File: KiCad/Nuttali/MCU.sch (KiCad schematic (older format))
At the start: 34 parts, among them J1 SWD, SW1 SW_DPST_x2, SW2 RND 210-00662, U1 STM32F411RETx, Y1 16Mhz

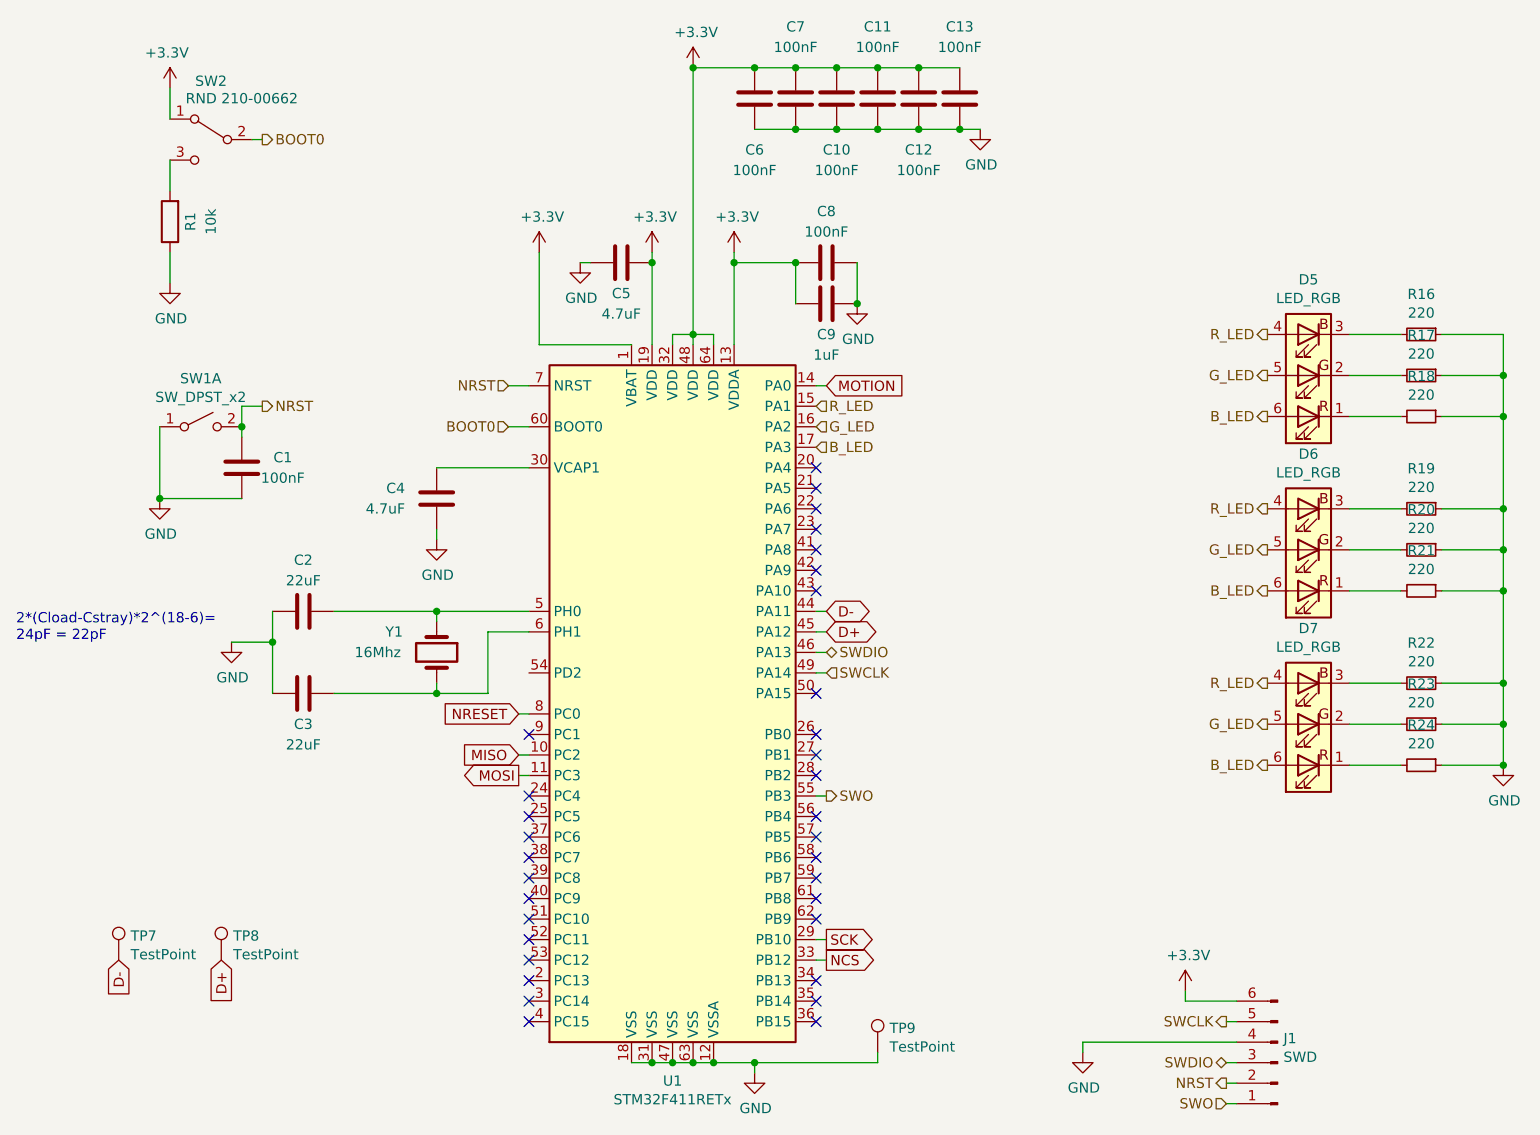
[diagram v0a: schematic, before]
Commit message: First draft of the pcb
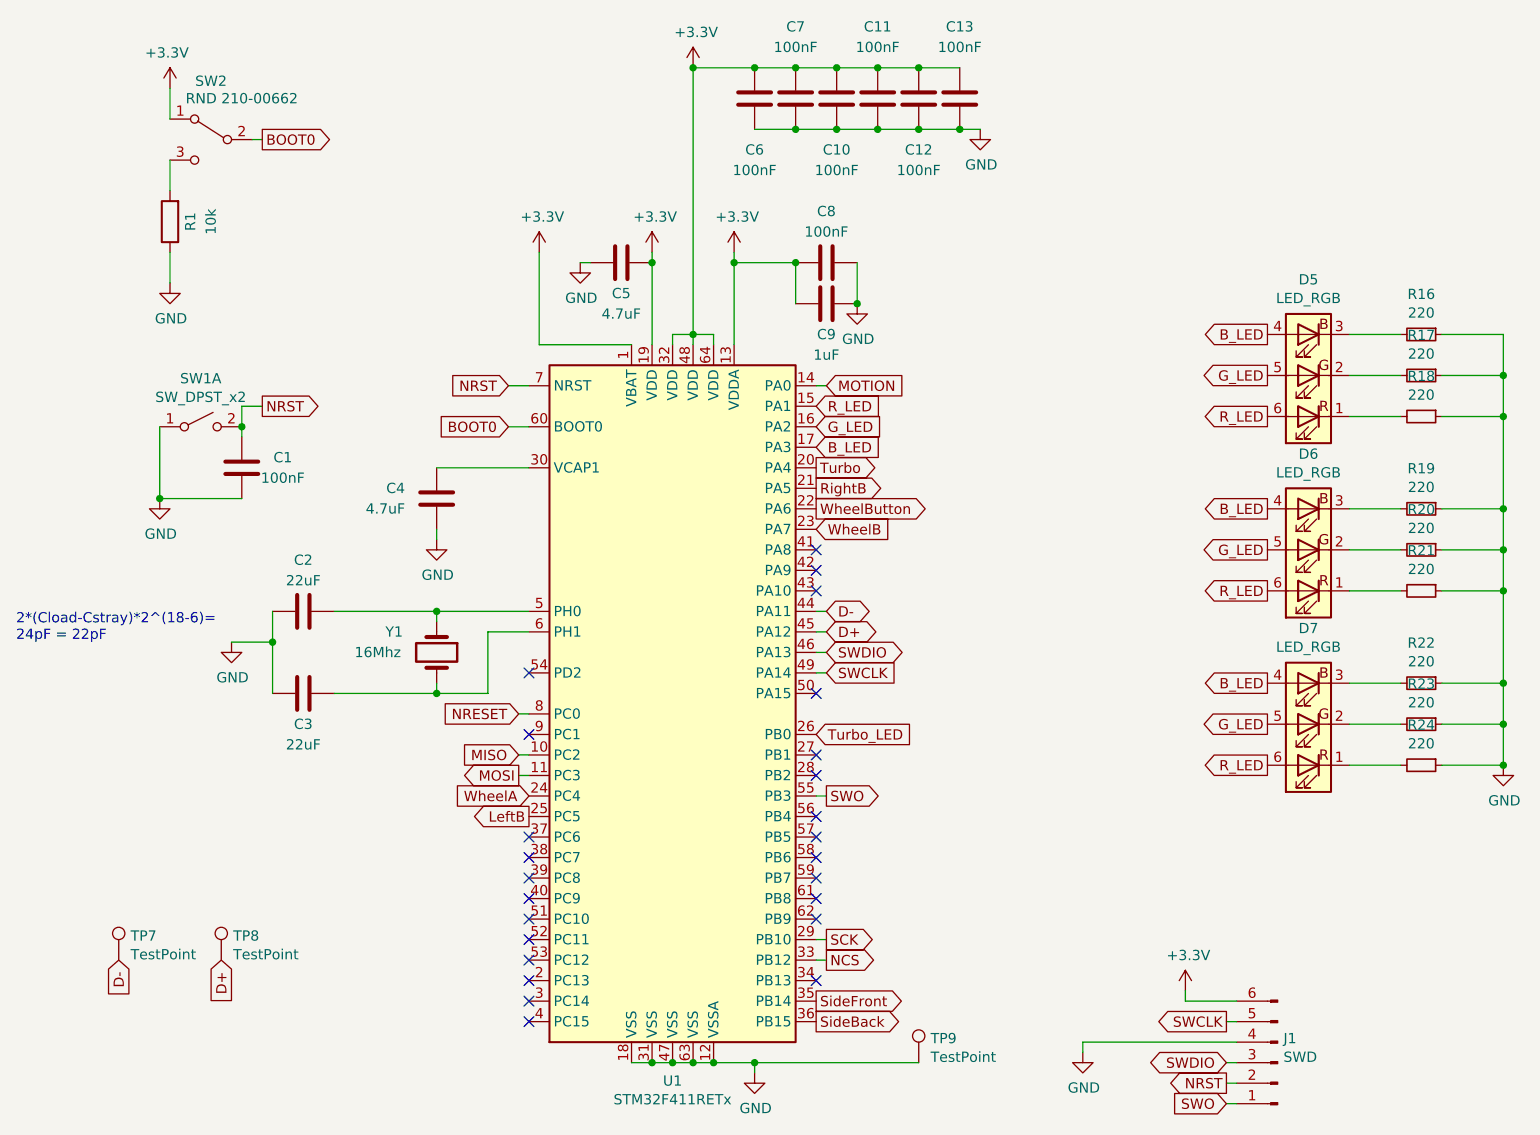
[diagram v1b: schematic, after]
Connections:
- net B_LED: now also D5.4 (BA), D6.4 (BA), D7.4 (BA); no longer D5.6 (RA), D6.6 (RA), D7.6 (RA)
- net R_LED: now also D5.6 (RA), D6.6 (RA), D7.6 (RA); no longer D5.4 (BA), D6.4 (BA), D7.4 (BA)
- net Turbo: now reaches U1.20 (PA4)
- net RightB: now reaches U1.21 (PA5)
- net WheelButton: now reaches U1.22 (PA6)
- net WheelB: now reaches U1.23 (PA7)
- net WheelA: now reaches U1.24 (PC4)
- net LeftB: now reaches U1.25 (PC5)
- net Turbo_LED: now reaches U1.26 (PB0)
- net SideFront: now reaches U1.35 (PB14)
- net SideBack: now reaches U1.36 (PB15)
- no-connect marks 33 -> 25
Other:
- moved on the sheet: TP9

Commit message: extended the pcb board with 2 mm to right
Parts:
- D5, D6, D7: symbol Device:LED_RGB -> Nuttali-rescue:LED_RGB-Device
- J1: symbol Connector:Conn_01x06_Male -> Nuttali-rescue:Conn_01x06_Male-Connector
- R1: symbol Device:R -> Nuttali-rescue:R-Device
- R16, R17, R18, R19, R20, R21, R22, R23, R24: symbol Device:R_Small -> Nuttali-rescue:R_Small-Device
- SW1: symbol Switch:SW_DPST_x2 -> Nuttali-rescue:SW_DPST_x2-Switch
- SW2: symbol Switch:SW_SPDT -> Nuttali-rescue:SW_SPDT-Switch
- TP7, TP8, TP9: symbol Connector:TestPoint -> Nuttali-rescue:TestPoint-Connector
- Y1: symbol Device:Crystal -> Nuttali-rescue:Crystal-Device
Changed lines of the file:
@@
 2*(Cload-Cstray)*2^(18-6)= \n24pF = 22pF
 $Comp
-L Device:Crystal Y1
+L Nuttali-rescue:Crystal-Device Y1
 U 1 1 602B614B
 P 4300 3950
@@
 	4650 2850 4750 2850
 $Comp
-L Connector:Conn_01x06_Male J1
+L Nuttali-rescue:Conn_01x06_Male-Connector J1
 U 1 1 602DCAE5
 P 8400 5950
@@
 $EndComp
 $Comp
-L Switch:SW_SPDT SW2
+L Nuttali-rescue:SW_SPDT-Switch SW2
 U 1 1 602EAC7D
 P 3200 1450
@@
 	3000 1550 3000 1700
 $Comp
-L Device:R R1
+L Nuttali-rescue:R-Device R1
 U 1 1 602EF78F
 P 3000 1850
@@
 	7950 5650 7950 5600
 $Comp
-L power:+3.3V #PWR0114
+L Nuttali-rescue:+3.3V-power #PWR0114
 U 1 1 601F634D
 P 7950 5600
@@
 $EndComp
 $Comp
-L power:GND #PWR0115
+L Nuttali-rescue:GND-power #PWR0115
 U 1 1 601F695B
 P 7450 5900
@@
 NoConn ~ 4750 4350
 $Comp
-L Switch:SW_DPST_x2 SW1
+L Nuttali-rescue:SW_DPST_x2-Switch SW1
 U 1 1 60245B0E
 P 3150 2850
@@
 	3350 2850 3350 2900
 $Comp
-L Connector:TestPoint TP9
+L Nuttali-rescue:TestPoint-Connector TP9
 U 1 1 60242CC3
 P 6650 5950
@@
 Connection ~ 5850 5950
 $Comp
-L Connector:TestPoint TP7
+L Nuttali-rescue:TestPoint-Connector TP7
 U 1 1 6024AE5A
 P 2750 5450
@@
 $EndComp
 $Comp
-L Connector:TestPoint TP8
+L Nuttali-rescue:TestPoint-Connector TP8
 U 1 1 6024B3CD
 P 3250 5450
@@
 $EndComp
 $Comp
-L Device:R_Small R24
+L Nuttali-rescue:R_Small-Device R24
 U 1 1 6032C1C8
 P 9100 4500
@@
 $EndComp
 $Comp
-L Device:R_Small R23
+L Nuttali-rescue:R_Small-Device R23
 U 1 1 6032C1C2
 P 9100 4300
@@
 $EndComp
 $Comp
-L Device:R_Small R22
+L Nuttali-rescue:R_Small-Device R22
 U 1 1 6032C1BC
 P 9100 4100
@@
 $EndComp
 $Comp
-L Device:R_Small R21
+L Nuttali-rescue:R_Small-Device R21
 U 1 1 60329EB6
 P 9100 3650
@@
 $EndComp
 $Comp
-L Device:R_Small R20
+L Nuttali-rescue:R_Small-Device R20
 U 1 1 60329EB0
 P 9100 3450
@@
 $EndComp
 $Comp
-L Device:R_Small R19
+L Nuttali-rescue:R_Small-Device R19
 U 1 1 60329EAA
 P 9100 3250
@@
 $EndComp
 $Comp
-L Device:R_Small R18
+L Nuttali-rescue:R_Small-Device R18
 U 1 1 60327306
 P 9100 2800
@@
 $EndComp
 $Comp
-L Device:R_Small R17
+L Nuttali-rescue:R_Small-Device R17
 U 1 1 60326D05
 P 9100 2600
@@
 $EndComp
 $Comp
-L Device:R_Small R16
+L Nuttali-rescue:R_Small-Device R16
 U 1 1 6032557E
 P 9100 2400
@@
 $EndComp
 $Comp
-L Device:LED_RGB D5
+L Nuttali-rescue:LED_RGB-Device D5
 U 1 1 60285E04
 P 8550 2600
@@
 $EndComp
 $Comp
-L Device:LED_RGB D6
+L Nuttali-rescue:LED_RGB-Device D6
 U 1 1 602851F0
 P 8550 3450
@@
 $EndComp
 $Comp
-L Device:LED_RGB D7
+L Nuttali-rescue:LED_RGB-Device D7
 U 1 1 6028314D
 P 8550 4300

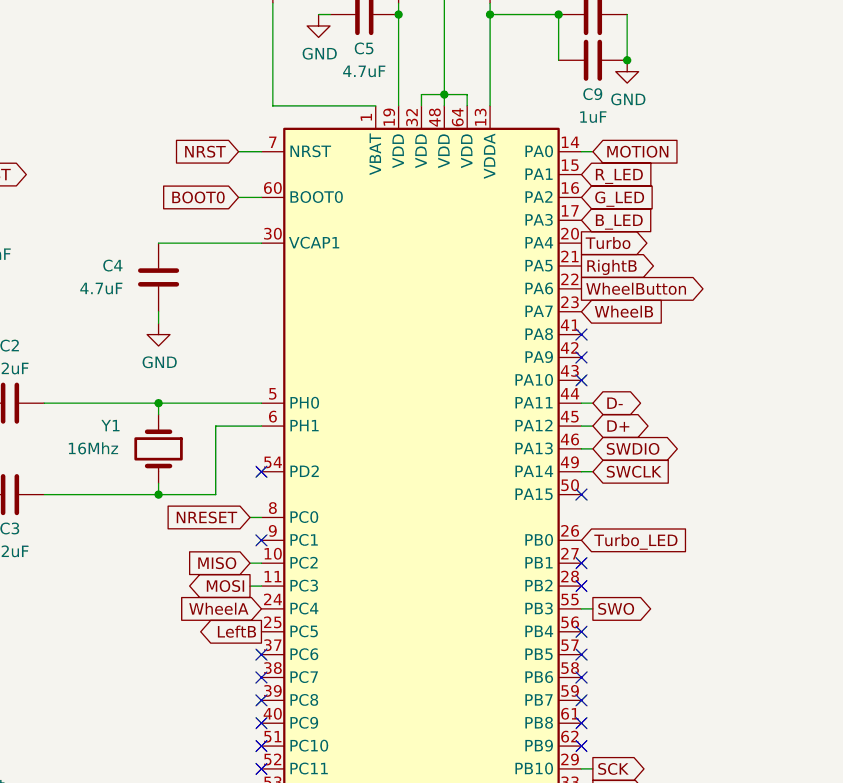
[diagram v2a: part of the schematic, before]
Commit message: Finnished the pcb
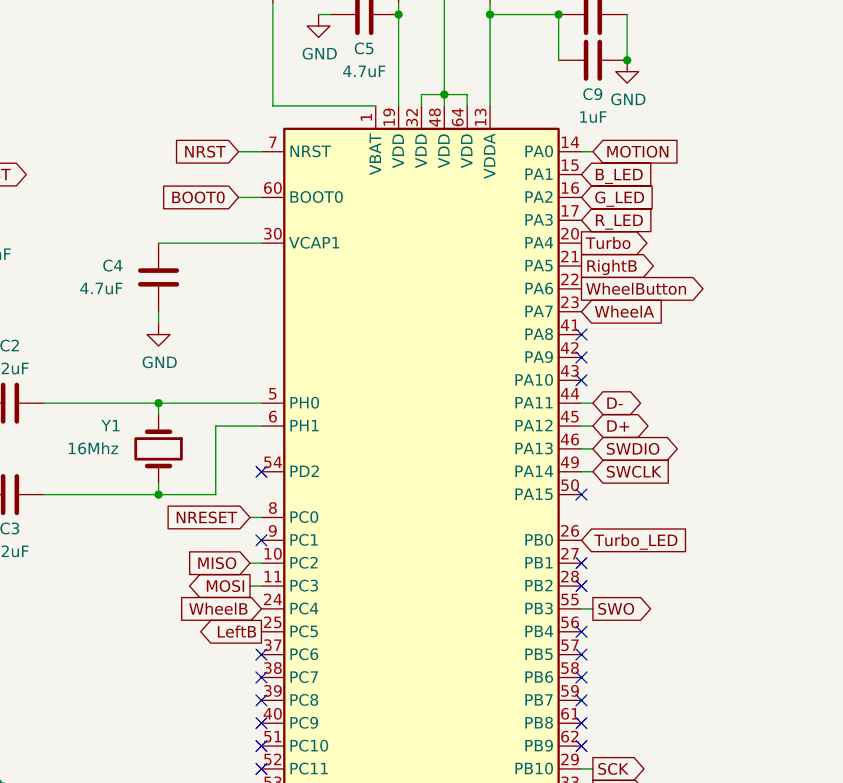
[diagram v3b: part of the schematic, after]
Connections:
- net B_LED: now also U1.15 (PA1); no longer U1.17 (PA3)
- net R_LED: now also U1.17 (PA3); no longer U1.15 (PA1)
- net WheelA: now also U1.23 (PA7); no longer U1.24 (PC4)
- net WheelB: now also U1.24 (PC4); no longer U1.23 (PA7)
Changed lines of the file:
@@
 Text GLabel 4650 2850 0    50   Input ~ 0
 BOOT0
-Text GLabel 6150 2750 2    50   Input ~ 0
+Text GLabel 6150 2950 2    50   Input ~ 0
 R_LED
 Text GLabel 6150 2850 2    50   Input ~ 0
 G_LED
-Text GLabel 6150 2950 2    50   Input ~ 0
-B_LED
 Text GLabel 8350 2800 0    50   Output ~ 0
 R_LED
@@
 Text GLabel 6150 4350 2    50   Input ~ 0
 Turbo_LED
-Text GLabel 6150 3050 2    50   Output ~ 0
-Turbo
-Text GLabel 6150 3350 2    50   Input ~ 0
+Text GLabel 4750 4650 0    50   Input ~ 0
 WheelB
-Text GLabel 4750 4650 0    50   Input ~ 0
-WheelA
 Text GLabel 6150 3250 2    50   Output ~ 0
 WheelButton
@@
 Text GLabel 4750 4750 0    50   Output ~ 0
 LeftB
-Text GLabel 6150 3150 2    50   Output ~ 0
-RightB
 NoConn ~ 6150 3450
 NoConn ~ 6150 3550
@@
 Wire Wire Line
 	5850 5950 6650 5950
+Text GLabel 6150 3050 2    50   Output ~ 0
+Turbo
+Text GLabel 6150 2750 2    50   Input ~ 0
+B_LED
+Text GLabel 6150 3150 2    50   Output ~ 0
+RightB
+Text GLabel 6150 3350 2    50   Input ~ 0
+WheelA
 $EndSCHEMATC
